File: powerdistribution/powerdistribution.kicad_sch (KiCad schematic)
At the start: 126 parts, among them IC1 NCP718ASNADJT1G, J1 282837-2, J2 282837-2, J3 M20-6102045, Q1 IRLML0030, Q2 IRLML0030, Q3 IRLML0030, Q5 IRLML0030, U1 BQ7790512PW, U2 AP64501QSP-13, U3 AP64501QSP-13, U4 AP64501QSP-13, U5 TPS1HC30BQPWPRQ1, U6 TPS1HC30BQPWPRQ1, U7 ESP32-DEVKIT-V1, U8 LD1117S50TR_SOT223, U9 MIC29302AWD-TR

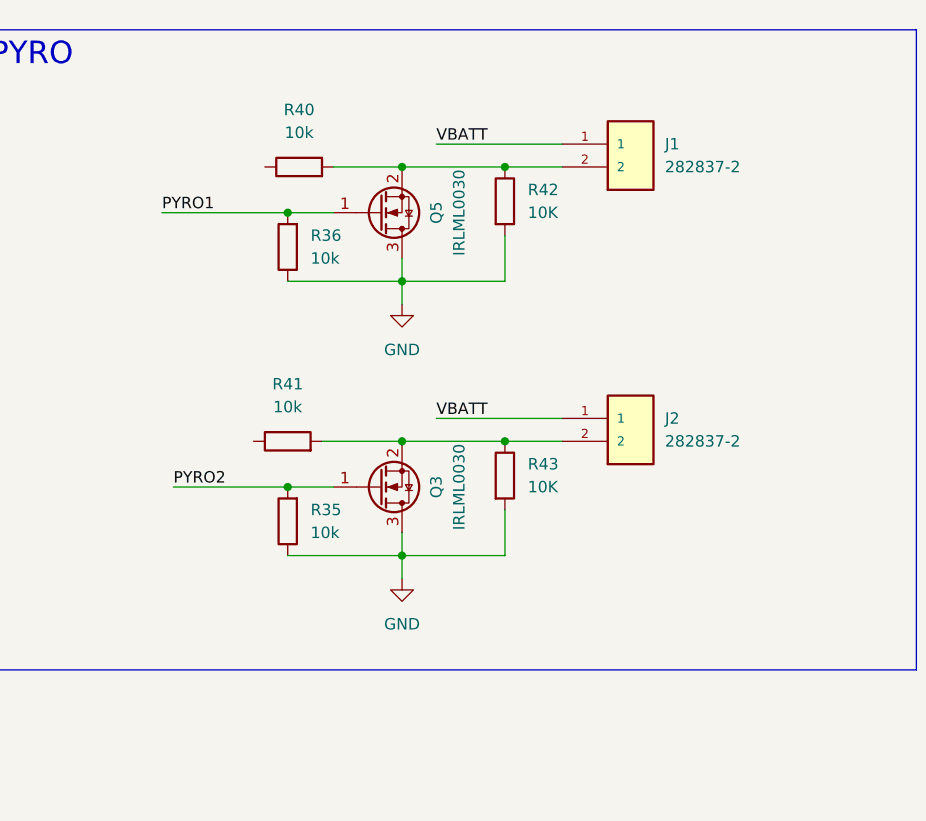
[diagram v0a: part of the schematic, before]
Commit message: updated pyro
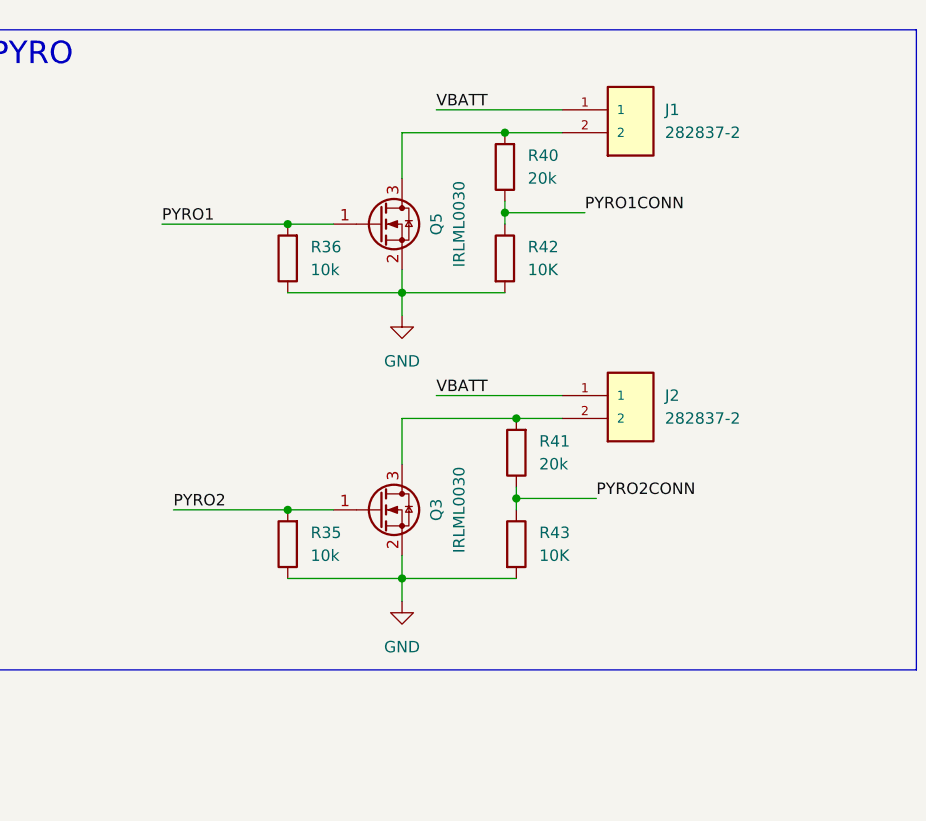
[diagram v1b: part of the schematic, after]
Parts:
- R40, R41: value 10k -> 20k
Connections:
- net GND: now also Q3.2 (S), Q5.2 (S); no longer Q3.3 (D), Q5.3 (D)
- net PYRO2CONN: now reaches R41.1
- net PYRO2CONN: now also R43.1
- net at J2.2, R41.2: now also Q3.3 (D); no longer Q3.2 (S), R43.1
- net at J1.2, R40.2: now also Q5.3 (D); no longer Q5.2 (S), R42.1
- net PYRO1CONN: now reaches R40.1
- net PYRO1CONN: now also R42.1
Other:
- moved on the sheet: J1, J2, Q3, Q5, R35, R36, R40, R41, R42, R43
